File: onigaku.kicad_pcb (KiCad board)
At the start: 2 copper layers, 333.9 x 110.2 mm, 312 parts, among them J1 MJ-4PP-9, J2 MJ-4PP-9, U1 Elite-C, U2 Elite-C

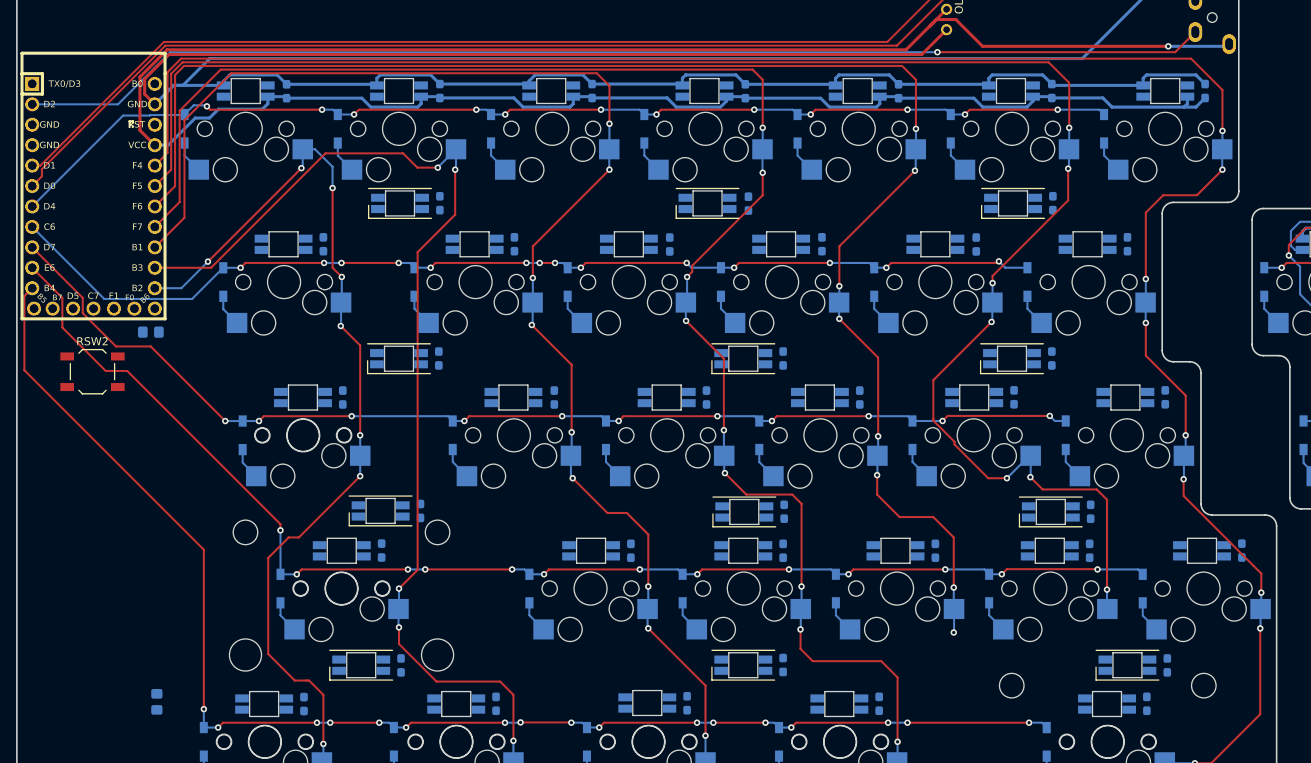
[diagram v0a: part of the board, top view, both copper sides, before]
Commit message: created more traces on left, all grounds first pass
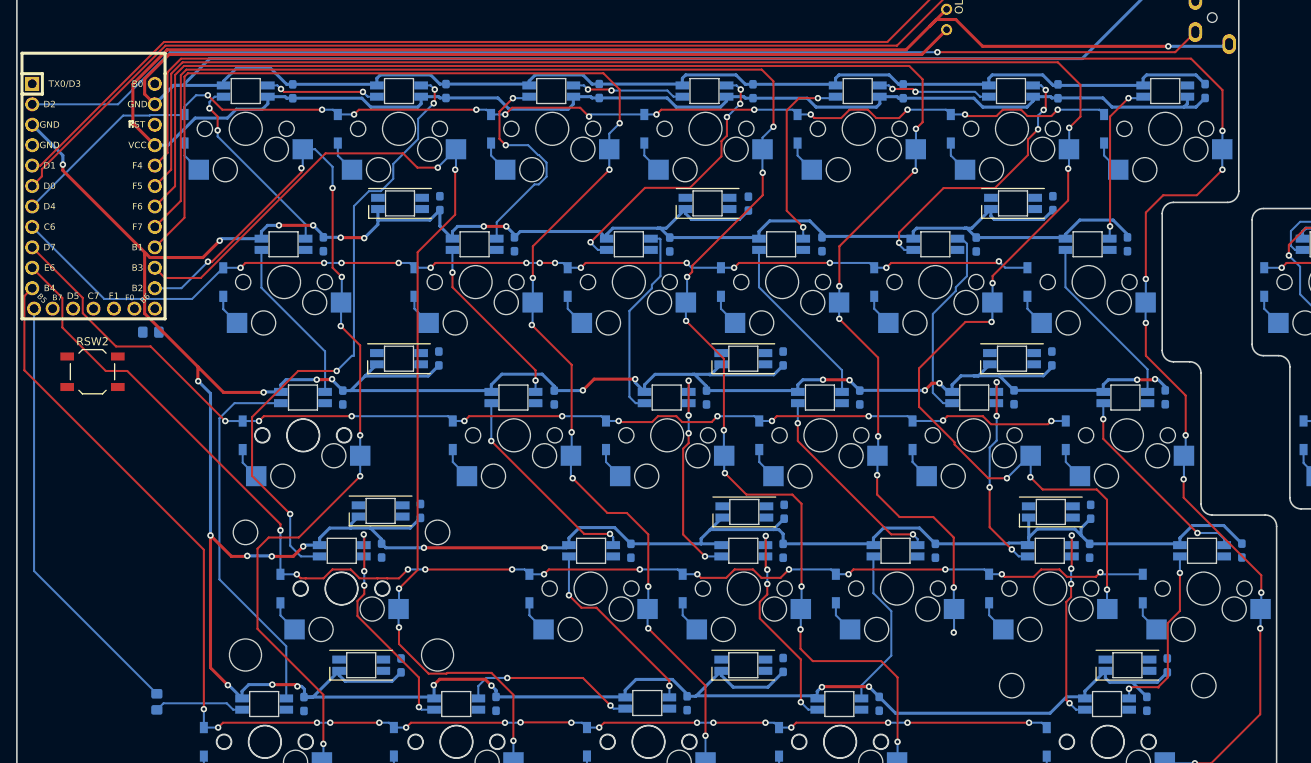
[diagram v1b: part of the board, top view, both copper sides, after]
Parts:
- moved C30 0.95 mm to (214.2, 161.8)
- moved C35 0.89 mm to (195.1, 161.8)
- moved C32 0.76 mm to (252.1, 161.8)
- moved C36 0.76 mm to (157.0, 161.8)
- moved C34 0.76 mm to (176.0, 161.8)
- moved C31 0.57 mm to (232.9, 161.8)
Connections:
- LED85 pad 2: Net-(LED73-Pad4) -> Net-(LED75-Pad4)
- LED85 pad 4: Net-(LED84-Pad2) -> Net-(LED74-Pad2)
- LED86 pad 2: Net-(LED86-Pad2) -> Net-(LED73-Pad4)
- LED86 pad 4: Net-(LED74-Pad2) -> Net-(LED84-Pad2)
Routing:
- net GND: track 380.8 -> 1134.2 mm, vias 0 -> 33
- net Net-(LED33-Pad2): track 0.00 -> 78.0 mm, vias 0 -> 4
- net LED_L: track 0.00 -> 54.2 mm
- net Net-(LED60-Pad4): track 0.00 -> 46.7 mm
- net Net-(LED35-Pad2): track 0.00 -> 34.4 mm, vias 0 -> 4
- net Net-(LED37-Pad2): track 0.00 -> 34.3 mm, vias 0 -> 4
- net Net-(LED72-Pad2): track 0.00 -> 28.4 mm, vias 0 -> 4
- net Net-(LED34-Pad4): track 0.00 -> 27.2 mm, vias 0 -> 2
- net Net-(LED74-Pad2): track 0.00 -> 26.9 mm, vias 0 -> 4
- net Net-(LED62-Pad2): track 0.00 -> 26.7 mm, vias 0 -> 4
- net Net-(LED61-Pad4): track 0.00 -> 26.6 mm, vias 0 -> 2
- net Net-(LED64-Pad2): track 0.00 -> 25.8 mm, vias 0 -> 4
- net Net-(LED76-Pad2): track 0.00 -> 25.5 mm, vias 0 -> 4
- net Net-(LED63-Pad4): track 0.00 -> 25.4 mm, vias 0 -> 2
- net Net-(LED65-Pad4): track 0.00 -> 25.4 mm, vias 0 -> 2
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
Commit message: adding fill areas
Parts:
- removed C19, C9: 0.1uF, Capacitor_SMD:C_0603_1608Metric_Pad1.08x0.95mm_HandSolder
- removed LED11, LED20: YS-SK6812MINI-E, kbd:YS-SK6812MINI-E_underglow
- moved C21 0.95 mm to (266.6, 233.2)
- moved J2 0.39 mm to (289.4, 144.3)
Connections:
- LED12 pad 4: Net-(LED11-Pad2) -> Net-(LED12-Pad4)
- LED19 pad 2: Net-(LED19-Pad2) -> Net-(LED12-Pad4)
- LED21 pad 2: Net-(LED20-Pad4) -> Net-(LED21-Pad2)
- LED21 pad 4: Net-(LED21-Pad4) -> Net-(LED10-Pad2)
- LED22 pad 2: Net-(LED21-Pad4) -> Net-(LED22-Pad2)
- LED22 pad 4: Net-(LED22-Pad4) -> Net-(LED21-Pad2)
- LED23 pad 2: Net-(LED22-Pad4) -> Net-(LED23-Pad2)
- LED23 pad 4: Net-(LED23-Pad4) -> Net-(LED22-Pad2)
- LED24 pad 2: Net-(LED23-Pad4) -> Net-(LED19-Pad4)
- LED24 pad 4: Net-(LED12-Pad2) -> Net-(LED23-Pad2)
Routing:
- net VCC: track 296.7 -> 1277.5 mm, vias 1 -> 42
- net GND: track 1134.2 -> 974.8 mm, vias 33 -> 24
- net GNDA: track 1201.6 -> 1079.4 mm, vias 63 -> 24
- net Net-(LED22-Pad2): track 0.00 -> 65.3 mm, vias 0 -> 6
- net Net-(LED23-Pad2): track 0.00 -> 62.2 mm, vias 0 -> 6
- net Net-(LED19-Pad4): track 0.00 -> 45.0 mm, vias 0 -> 6
- net Net-(LED7-Pad4): track 0.00 -> 42.5 mm, vias 0 -> 2
- net reset_L: track 0.00 -> 37.0 mm, vias 0 -> 3
- net Net-(LED8-Pad2): track 0.00 -> 35.9 mm, vias 0 -> 2
- net Net-(LED7-Pad2): track 0.00 -> 35.0 mm, vias 0 -> 2
- net Net-(LED12-Pad4): track 0.00 -> 27.1 mm, vias 0 -> 2
- net Net-(LED21-Pad2): track 0.00 -> 21.9 mm, vias 0 -> 4
- net Net-(LED10-Pad4): track 0.00 -> 20.3 mm, vias 0 -> 2
- net Net-(LED10-Pad2): track 0.00 -> 18.8 mm, vias 0 -> 4
- net row1_L: track 131.7 -> 145.3 mm, vias 14 -> 16
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- added copper zone on B.Cu, net GND
- added copper zone on B.Cu, net GNDA

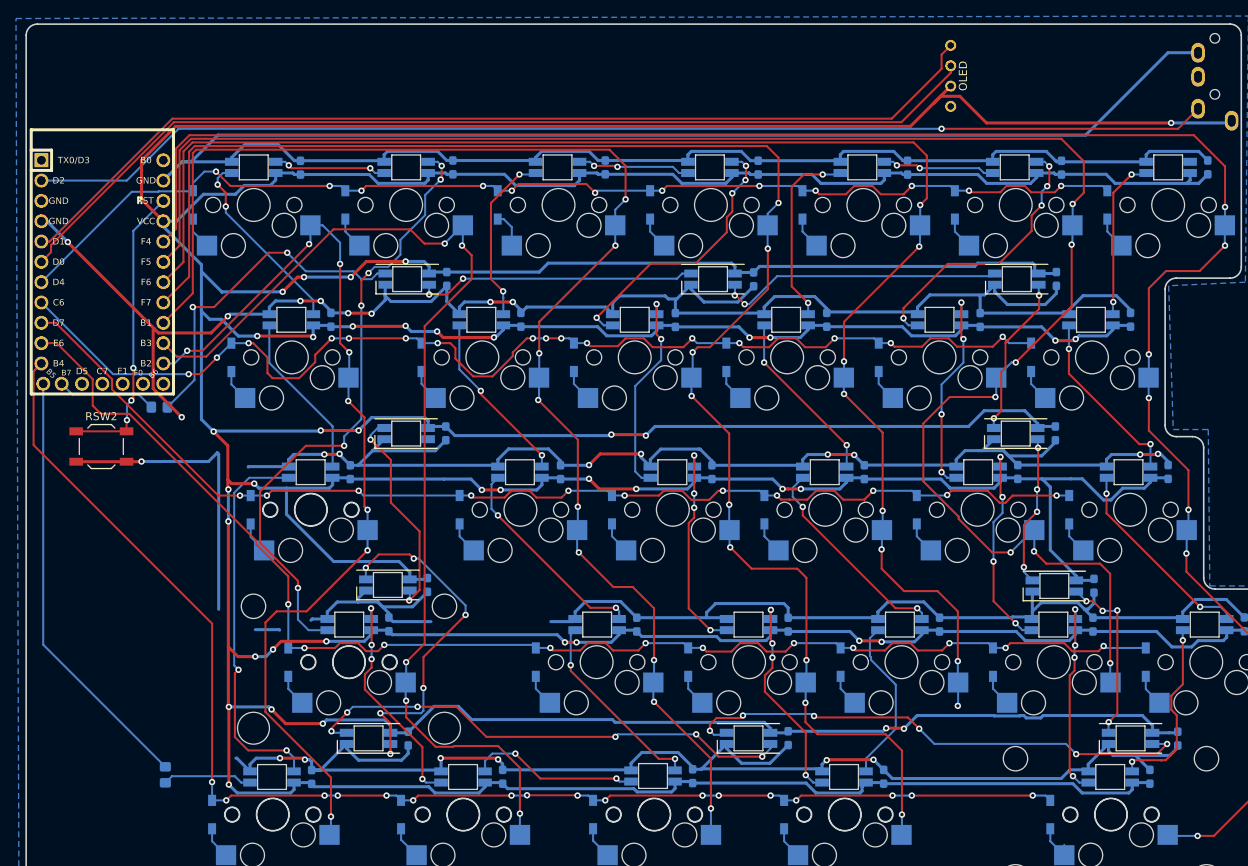
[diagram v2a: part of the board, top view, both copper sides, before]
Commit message: rewiring to make traces more readable
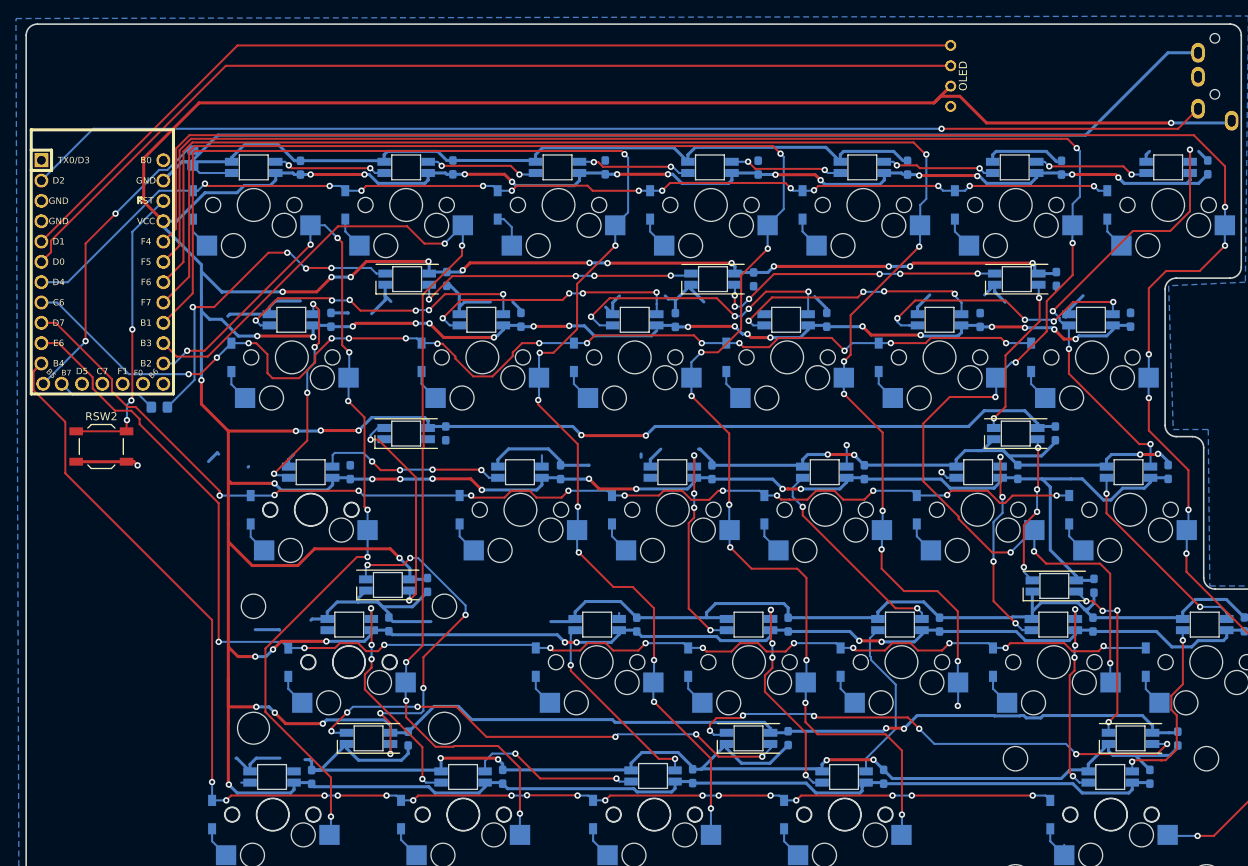
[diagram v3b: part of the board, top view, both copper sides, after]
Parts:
- moved R4 77.2 mm to (143.5, 160.6)
- turned C30 to 90 degrees
- turned C31 to 90 degrees
- turned C34 to 90 degrees
- turned C35 to 90 degrees
- turned C57 to 90 degrees
- turned C58 to 90 degrees
- turned C59 to 90 degrees
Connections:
- C30 pad 1: GND -> VCC
- C30 pad 2: VCC -> GND
- C31 pad 1: GND -> VCC
- C31 pad 2: VCC -> GND
- C34 pad 1: GND -> VCC
- C34 pad 2: VCC -> GND
- C35 pad 1: GND -> VCC
- C35 pad 2: VCC -> GND
- C57 pad 1: GND -> VCC
- C57 pad 2: VCC -> GND
- C58 pad 1: GND -> VCC
- C58 pad 2: VCC -> GND
- C59 pad 1: GND -> VCC
- C59 pad 2: VCC -> GND
- C60 pad 1: GND -> VCC
- C60 pad 2: VCC -> GND
- C61 pad 1: GND -> VCC
- C61 pad 2: VCC -> GND
- C68 pad 1: GND -> VCC
- C68 pad 2: VCC -> GND
- C69 pad 1: GND -> VCC
- C69 pad 2: VCC -> GND
- C70 pad 1: GND -> VCC
- C70 pad 2: VCC -> GND
- C71 pad 1: GND -> VCC
- C71 pad 2: VCC -> GND
- C72 pad 1: GND -> VCC
- C72 pad 2: VCC -> GND
- C79 pad 1: GND -> VCC
- C79 pad 2: VCC -> GND
- C80 pad 1: GND -> VCC
- C80 pad 2: VCC -> GND
- C82 pad 1: GND -> VCC
- C82 pad 2: VCC -> GND
- C84 pad 1: GND -> VCC
- C84 pad 2: VCC -> GND
- C85 pad 1: GND -> VCC
- C85 pad 2: VCC -> GND
- LED34 pad 4: Net-(LED34-Pad4) -> Net-(LED33-Pad2)
- LED36 pad 4: Net-(LED36-Pad4) -> Net-(LED35-Pad2)
- LED38 pad 4: Net-(LED38-Pad4) -> Net-(LED37-Pad2)
- LED47 pad 2: Net-(LED32-Pad4) -> Net-(LED47-Pad2)
- LED48 pad 2: Net-(LED34-Pad4) -> Net-(LED47-Pad4)
- LED49 pad 2: Net-(LED49-Pad2) -> Net-(LED48-Pad4)
- LED49 pad 4: Net-(LED35-Pad2) -> Net-(LED49-Pad4)
- LED50 pad 2: Net-(LED36-Pad4) -> Net-(LED49-Pad4)
- LED51 pad 2: Net-(LED51-Pad2) -> Net-(LED50-Pad4)
- LED51 pad 4: Net-(LED37-Pad2) -> Net-(LED51-Pad4)
- LED52 pad 2: Net-(LED38-Pad4) -> Net-(LED51-Pad4)
- LED52 pad 4: Net-(LED52-Pad4) -> Net-(LED38-Pad2)
- LED60 pad 2: Net-(LED47-Pad4) -> Net-(LED60-Pad2)
- LED60 pad 4: Net-(LED60-Pad4) -> Net-(LED47-Pad2)
- LED61 pad 2: Net-(LED48-Pad4) -> Net-(LED61-Pad2)
- LED61 pad 4: Net-(LED61-Pad4) -> Net-(LED60-Pad2)
- LED62 pad 4: Net-(LED49-Pad2) -> Net-(LED62-Pad4)
- LED63 pad 1: VCC -> Net-(LED63-Pad1)
- LED63 pad 2: Net-(LED50-Pad4) -> Net-(LED63-Pad2)
- LED63 pad 4: Net-(LED63-Pad4) -> Net-(LED62-Pad2)
- LED64 pad 4: Net-(LED51-Pad2) -> Net-(LED64-Pad4)
- LED65 pad 2: Net-(LED52-Pad4) -> Net-(LED65-Pad2)
- LED72 pad 4: Net-(LED33-Pad2) -> Net-(LED72-Pad4)
- LED73 pad 2: Net-(LED61-Pad4) -> Net-(LED72-Pad4)
- LED74 pad 2: Net-(LED74-Pad2) -> Net-(LED73-Pad4)
- LED74 pad 4: Net-(LED62-Pad2) -> Net-(LED74-Pad4)
- LED75 pad 2: Net-(LED63-Pad4) -> Net-(LED74-Pad4)
- LED76 pad 2: Net-(LED76-Pad2) -> Net-(LED75-Pad4)
- LED76 pad 4: Net-(LED64-Pad2) -> Net-(LED76-Pad4)
- LED77 pad 2: Net-(LED65-Pad4) -> Net-(LED76-Pad4)
- LED77 pad 4: Net-(LED77-Pad4) -> Net-(LED65-Pad2)
- LED83 pad 2: Net-(LED60-Pad4) -> Net-(LED83-Pad2)
- LED83 pad 4: Net-(LED83-Pad4) -> Net-(LED72-Pad2)
- LED84 pad 4: Net-(LED72-Pad2) -> Net-(LED83-Pad2)
- LED85 pad 2: Net-(LED75-Pad4) -> Net-(LED85-Pad2)
- LED85 pad 4: Net-(LED74-Pad2) -> Net-(LED85-Pad4)
- LED86 pad 2: Net-(LED73-Pad4) -> Net-(LED85-Pad4)
- LED87 pad 2: Net-(LED77-Pad4) -> Net-(LED87-Pad2)
- LED87 pad 4: Net-(LED76-Pad2) -> Net-(LED85-Pad2)
- R4 pad 1: Net-(LED83-Pad4) -> Net-(LED32-Pad4)
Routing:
- net GND: track 974.8 -> 710.1 mm, vias 24 -> 9
- net Net-(LED33-Pad2): track 78.0 -> 14.2 mm, vias 6 -> 2
- net Net-(LED60-Pad4): track 48.7 -> 0.00 mm, vias 2 -> 0
- net Net-(LED49-Pad4): track 0.00 -> 36.3 mm, vias 0 -> 4
- net Net-(LED51-Pad4): track 0.00 -> 34.9 mm, vias 0 -> 4
- net Net-(LED38-Pad2): track 0.00 -> 34.0 mm, vias 0 -> 2
- net Net-(LED47-Pad2): track 0.00 -> 27.3 mm, vias 0 -> 4
- net Net-(LED61-Pad4): track 27.2 -> 0.00 mm, vias 2 -> 0
- net Net-(LED51-Pad2): track 26.6 -> 0.00 mm, vias 4 -> 0
- net Net-(LED49-Pad2): track 26.0 -> 0.00 mm, vias 2 -> 0
- net Net-(LED60-Pad2): track 0.00 -> 23.7 mm, vias 0 -> 4
- net Net-(LED36-Pad4): track 23.6 -> 0.00 mm, vias 2 -> 0
- net Net-(LED34-Pad4): track 21.7 -> 0.00 mm, vias 2 -> 0
- net Net-(LED38-Pad4): track 20.3 -> 0.00 mm, vias 2 -> 0
- net Net-(LED35-Pad2): track 34.4 -> 14.4 mm, vias 4 -> 2
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
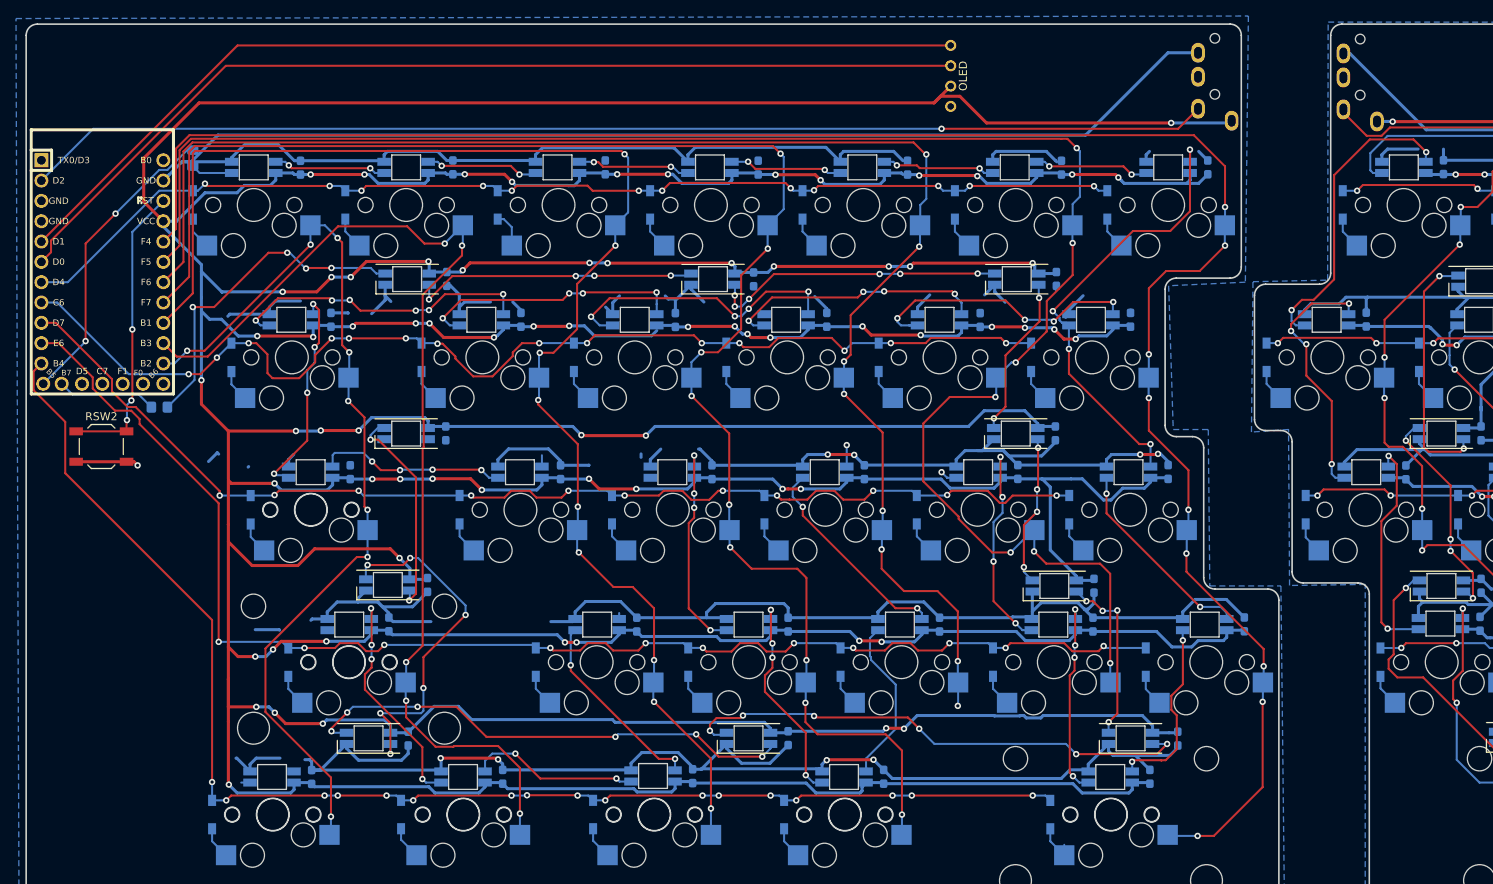
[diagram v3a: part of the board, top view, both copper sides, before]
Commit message: left side redone. wip on right side and whether or not to add nav section
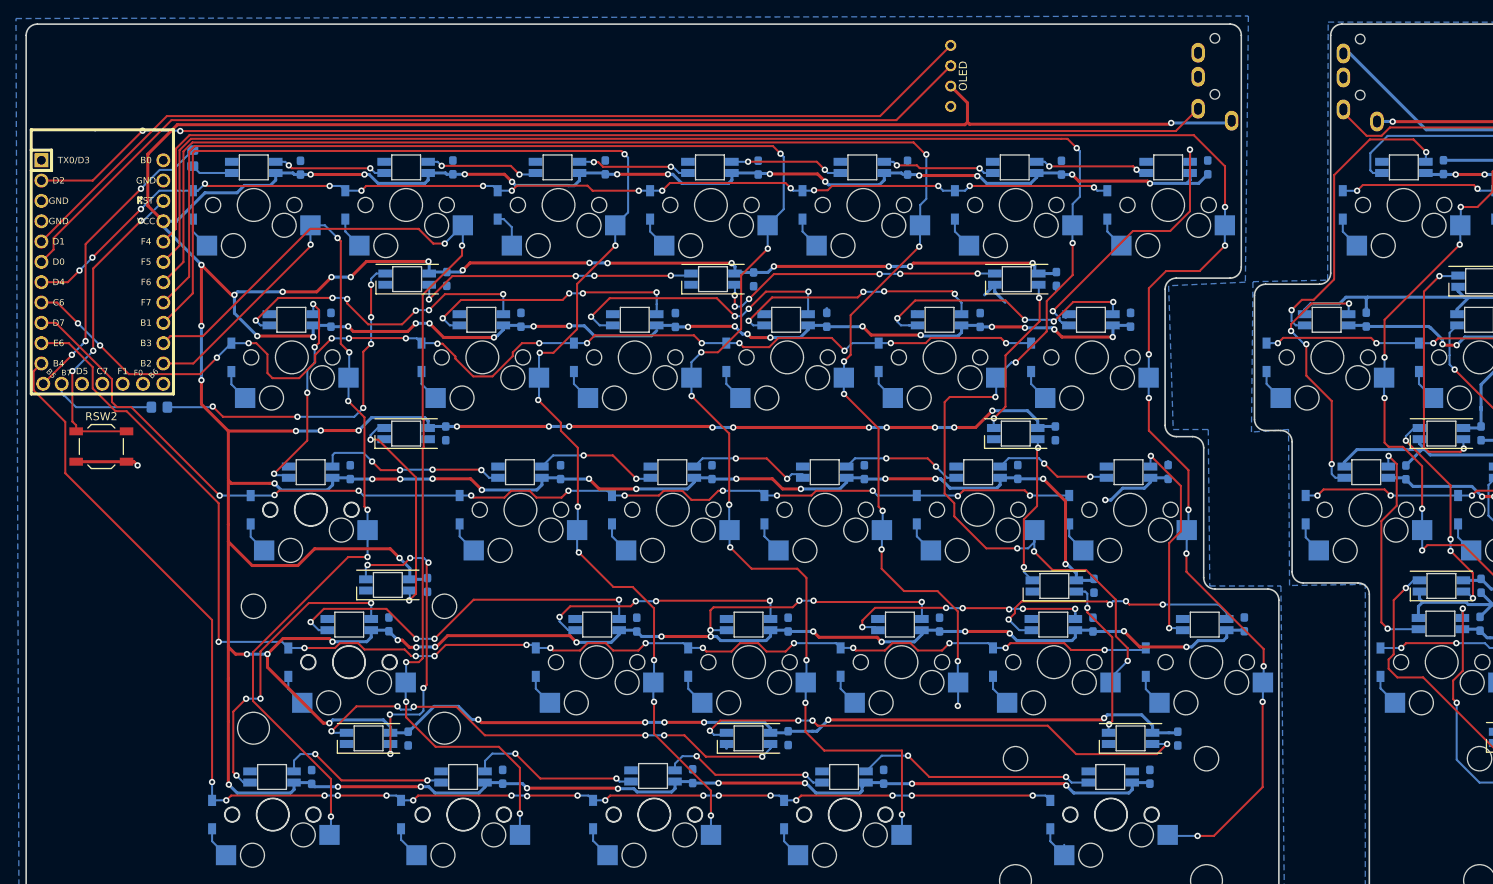
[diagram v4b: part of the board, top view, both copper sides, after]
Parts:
- turned C60 to 90 degrees
- turned C61 to 90 degrees
- turned C68 to 90 degrees
- turned C69 to 90 degrees
- turned C70 to 90 degrees
- turned C71 to 90 degrees
- turned C72 to 90 degrees
- turned C79 to 90 degrees
- turned C80 to 90 degrees
- turned C82 to 90 degrees
- turned C84 to 90 degrees
- turned C85 to 90 degrees
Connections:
- LED62 pad 4: Net-(LED62-Pad4) -> Net-(LED61-Pad2)
- LED63 pad 1: Net-(LED63-Pad1) -> VCC
- LED64 pad 4: Net-(LED64-Pad4) -> Net-(LED63-Pad2)
- LED65 pad 4: Net-(LED65-Pad4) -> Net-(LED64-Pad2)
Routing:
- net GND: track 710.1 -> 20.6 mm, vias 9 -> 1
- net Net-(LED72-Pad4): track 0.75 -> 47.7 mm, vias 0 -> 4
- net Net-(LED76-Pad4): track 0.00 -> 33.6 mm, vias 0 -> 4
- net Net-(LED74-Pad4): track 0.00 -> 33.6 mm, vias 0 -> 4
- net Net-(LED85-Pad2): track 0.00 -> 30.0 mm, vias 0 -> 2
- net Net-(LED74-Pad2): track 26.9 -> 0.00 mm, vias 4 -> 0
- net Net-(LED63-Pad4): track 26.4 -> 0.00 mm, vias 2 -> 0
- net Net-(LED65-Pad2): track 0.00 -> 26.4 mm, vias 0 -> 2
- net Net-(LED76-Pad2): track 25.5 -> 0.00 mm, vias 4 -> 0
- net Net-(LED65-Pad4): track 25.4 -> 0.00 mm, vias 2 -> 0
- net Net-(LED77-Pad4): track 24.1 -> 0.00 mm, vias 2 -> 0
- net Net-(LED52-Pad4): track 22.7 -> 0.00 mm, vias 2 -> 0
- net Net-(LED83-Pad2): track 0.00 -> 21.5 mm, vias 0 -> 2
- net Net-(LED85-Pad4): track 0.00 -> 21.0 mm, vias 0 -> 2
- net Net-(LED61-Pad2): track 1.42 -> 15.4 mm, vias 0 -> 2
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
